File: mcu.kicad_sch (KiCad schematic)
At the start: 20 parts, among them J1 Conn_01x04_Pin, J2 Conn_01x06_Pin, J3 Conn_01x04_Pin, SW1 SW_Nidec_CAS-120A1, SW2 SW_Push, U1 STM32G0B0KETx

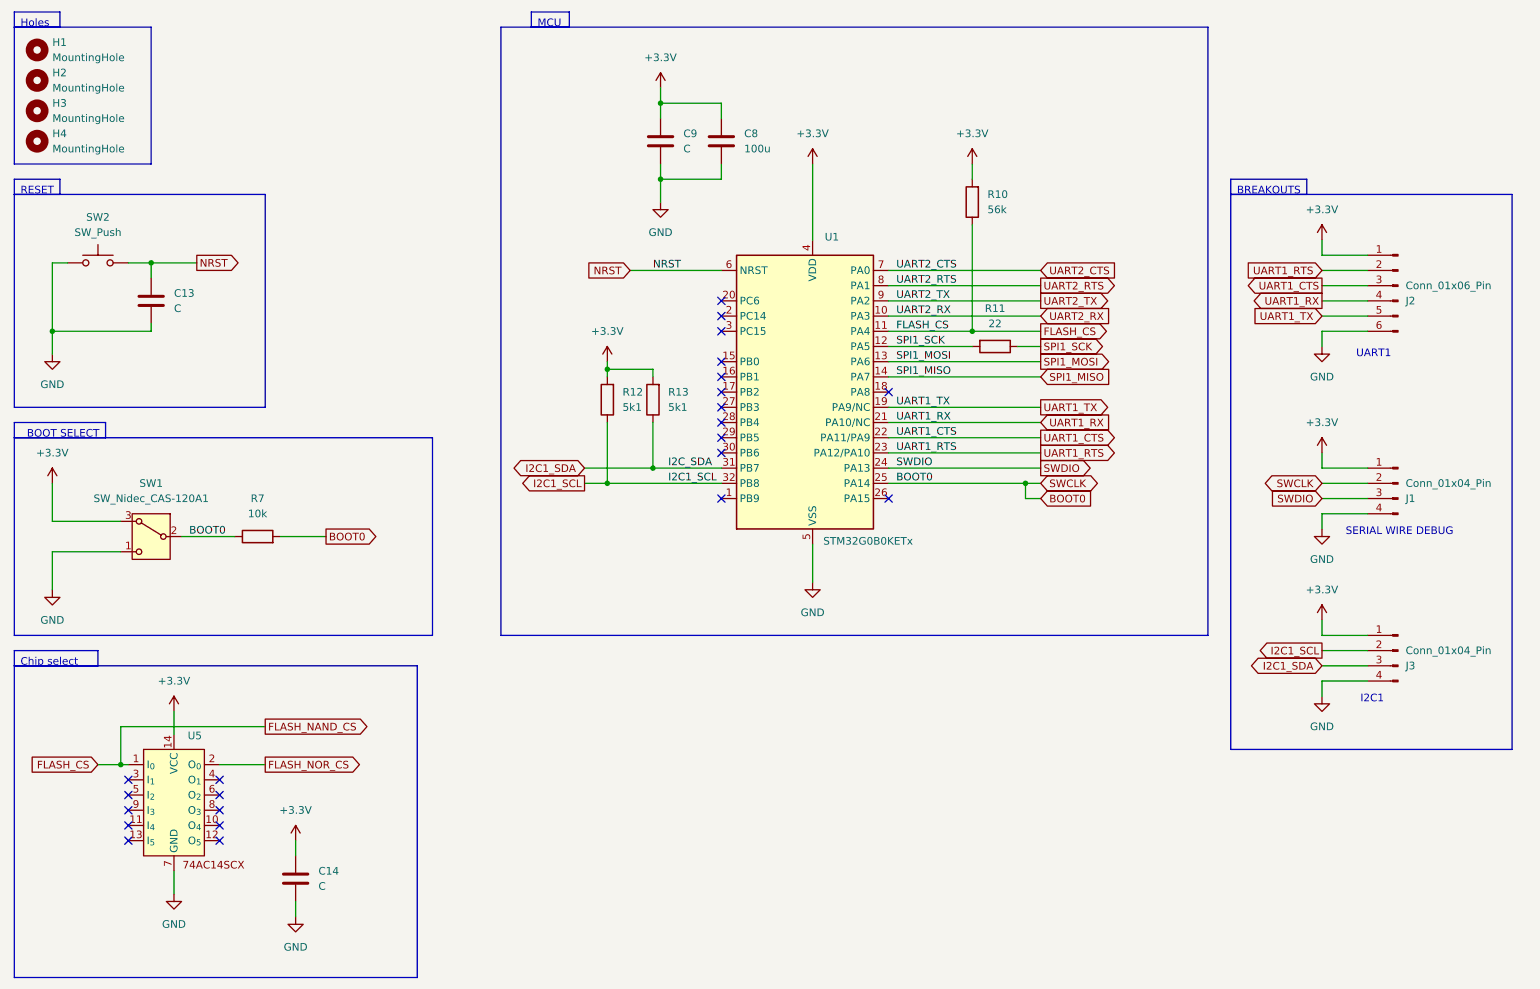
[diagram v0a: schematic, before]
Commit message: asdfsa
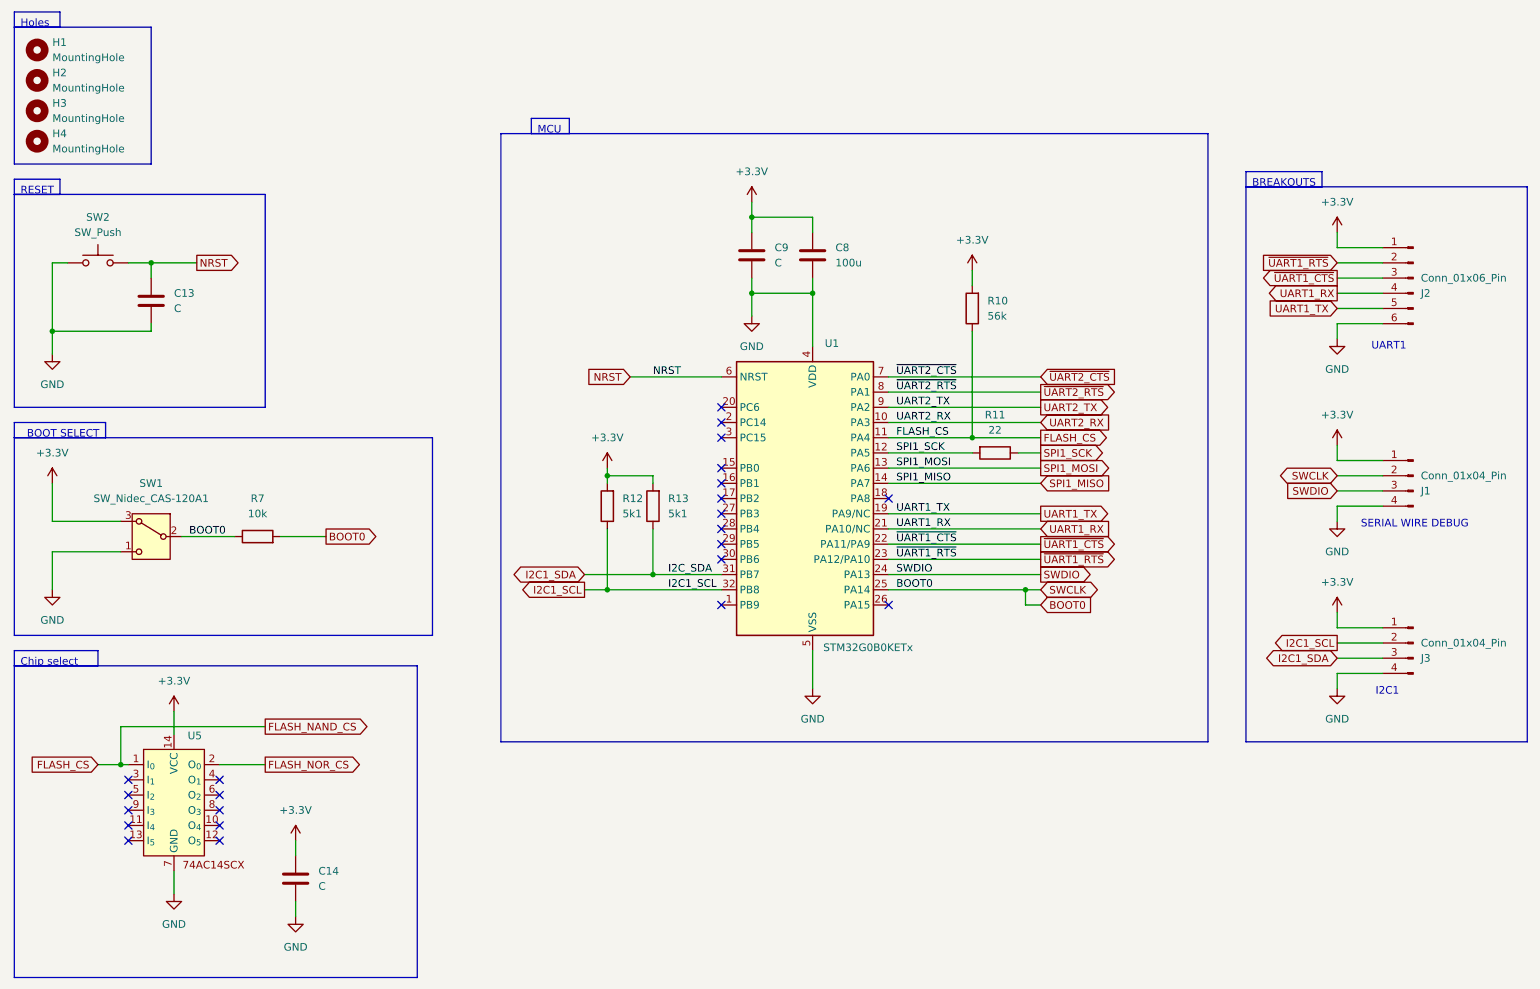
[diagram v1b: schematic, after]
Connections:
- net +3.3V: no longer U1.4 (VDD)
- net GND: now also U1.4 (VDD)
- net UART1_CTS renamed ~{UART1_CTS}
- net UART1_RTS renamed ~{UART1_RTS}
- net UART2_CTS renamed ~{UART2_CTS}
- net UART2_RTS renamed ~{UART2_RTS}
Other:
- moved on the sheet: C8, C9, J1, J2, J3, R10, R11, R12, R13, U1
